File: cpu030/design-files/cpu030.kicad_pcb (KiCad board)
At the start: 4 copper layers, 259.9 x 154.9 mm, 199 parts, among them J101 Reset, J102 SYSCTL JTAG, J103 NMI, J201 DRAM0SZ, J202 DRAM0 JTAG, J301 UART1 FTDI, J302 UART0 FTDI, J303 UART0, J304 UART1, J401 ISACTL JTAG, J501 ATA connector, J502 5V CF Power, J701 RJ45_Amphenol_RJMG1BD3B8K1ANR, J801 DIN41612_03x32_ABC, J901 ATX-24, SW101 Reset, SW102 NMI, U101 MC68030RC, U102 ATF1508AS, U103 MC74ACT05DG, U104 DS1813, U105 SST39SF040 (E), U106 SST39SF040 (O), U107 MC68882, U108 GAL22V10, U109 MC74ACT05DG, U110 DS1813, U201 ATF1508AS, U202 CY7C1061GE (U16), U203 CY7C1061GE (L16), U204 SIMM72-0A, U205 SIMM72-0B, U206 MC74ACT05DG, U301 TL16C2552, U401 ATF1508AS, U402 MC74ACT05DG, U501 74ACT245, U502 74ACT245, U503 74ACT245, U601 PCF8584, U602 DS3231MZ, U701 RTL8019AS, U702 AT93C46D-PU, U801 74ACT245, U802 74ACT245, U803 74ACT245, U804 74ACT245, U805 74ACT245, U806 74ACT245, U807 74ACT245, U808 74ACT245, Y101 50MHz, Y301 1.8432MHz, Y701 20MHz

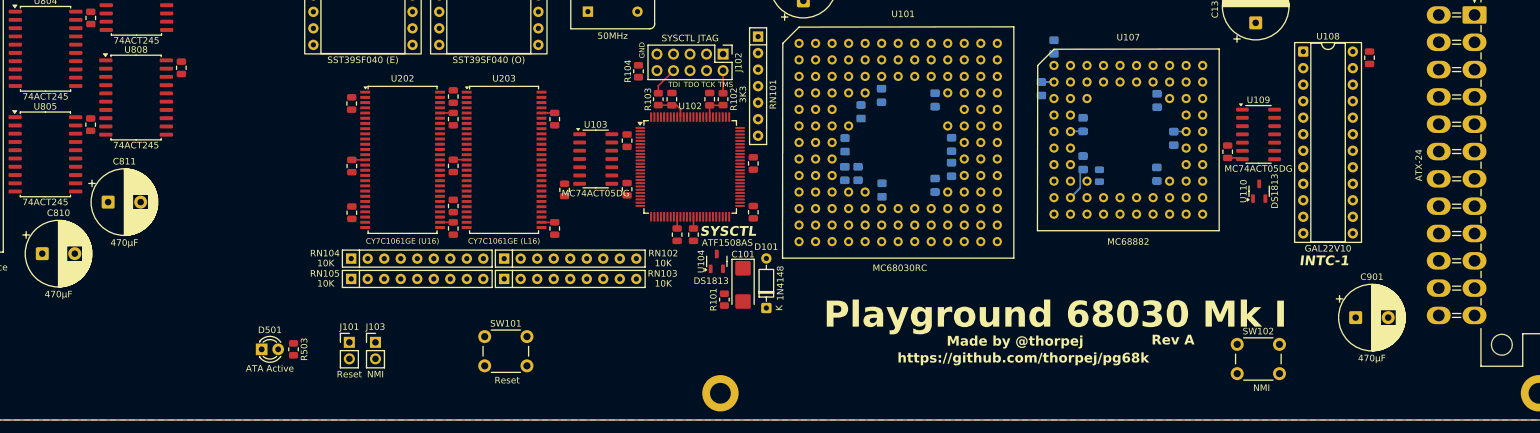
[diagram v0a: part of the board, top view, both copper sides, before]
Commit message: Manually route +12V and -12V.
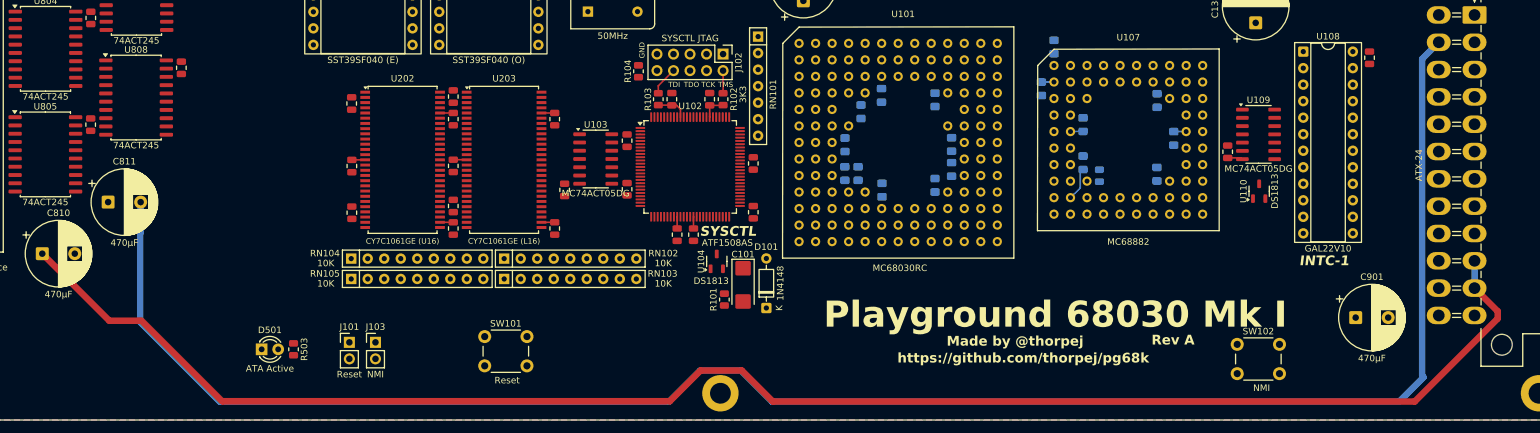
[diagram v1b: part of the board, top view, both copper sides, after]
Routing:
- net -12V: track 0.00 -> 279.0 mm
- net +12V: track 0.00 -> 252.5 mm
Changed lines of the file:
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@@
+	)
+	(segment
+		(start 224.2312 236.4994)
+		(end 219.4348 231.703)
+		(width 1)
+		(layer "B.Cu")
+		(net 429)
+	)
+	(segment
+		(start 139.2936 236.474)
+		(end 127.0762 224.2566)
+		(width 1)
+		(layer "B.Cu")
+		(net 429)
+	)
+	(segment
+		(start 324.172 232.5288)
+		(end 324.3834 232.7402)
+		(width 1)
+		(layer "B.Cu")
+		(net 429)
+	)
+	(segment
+		(start 127.143123 210.473677)
+		(end 127.143123 205.8162)
+		(width 1)
+		(layer "B.Cu")
+		(net 429)
+	)
+	(segment
+		(start 208.407 236.474)
+		(end 139.2936 236.474)
+		(width 1)
+		(layer "B.Cu")
+		(net 429)
+	)
+	(segment
+		(start 324.172 183.7916)
+		(end 324.172 232.5288)
+		(width 1)
+		(layer "B.Cu")
+		(net 429)
+	)
+	(segment
+		(start 127.0762 210.5406)
+		(end 127.143123 210.473677)
+		(width 1)
+		(layer "B.Cu")
+		(net 429)
+	)
+	(segment
+		(start 219.4348 231.703)
+		(end 213.178 231.703)
+		(width 1)
+		(layer "B.Cu")
+		(net 429)
+	)
+	(segment
+		(start 127.0762 224.2566)
+		(end 127.0762 210.5406)
+		(width 1)
+		(layer "B.Cu")
+		(net 429)
+	)
+	(segment
+		(start 213.178 231.703)
+		(end 208.407 236.474)
+		(width 1)
+		(layer "B.Cu")
+		(net 429)
+	)
+	(segment
+		(start 326.723 181.2406)
+		(end 324.172 183.7916)
+		(width 1)
+		(layer "B.Cu")
+		(net 429)
+	)
+	(segment
+		(start 320.6242 236.4994)
+		(end 224.2312 236.4994)
+		(width 1)
+		(layer "B.Cu")
+		(net 429)
+	)
+	(segment
+		(start 324.3834 232.7402)
+		(end 320.6242 236.4994)
+		(width 1)
+		(layer "B.Cu")
+		(net 429)
+	)
+	(segment
+		(start 127.1524 224.0534)
+		(end 122.3302 224.0534)
+		(width 1)
+		(layer "F.Cu")
+		(net 431)
+	)
+	(segment
+		(start 219.5618 231.703)
+		(end 213.2288 231.703)
+		(width 1)
+		(layer "F.Cu")
+		(net 431)
+	)
+	(segment
+		(start 335.7118 223.7994)
+		(end 323.0372 236.474)
+		(width 1)
+		(layer "F.Cu")
+		(net 431)
+	)
+	(segment
+		(start 208.5086 236.4232)
+		(end 139.7508 236.4232)
+		(width 1)
+		(layer "F.Cu")
+		(net 431)
+	)
+	(segment
+		(start 224.3328 236.474)
+		(end 219.5618 231.703)
+		(width 1)
+		(layer "F.Cu")
+		(net 431)
+	)
+	(segment
+		(start 335.788 222.6056)
+		(end 335.788 223.7232)
+		(width 1)
+		(layer "F.Cu")
+		(net 431)
+	)
+	(segment
+		(start 213.2288 231.703)
+		(end 208.5086 236.4232)
+		(width 1)
+		(layer "F.Cu")
+		(net 431)
+	)
+	(segment
+		(start 323.0372 236.474)
+		(end 224.3328 236.474)
+		(width 1)
+		(layer "F.Cu")
+		(net 431)
+	)
+	(segment
+		(start 139.7 236.474)
+		(end 127.2794 224.0534)
+		(width 1)
+		(layer "F.Cu")
+		(net 431)
+	)
+	(segment
+		(start 122.3302 224.0534)
+		(end 112.0178 213.741)
+		(width 1)
+		(layer "F.Cu")
+		(net 431)
+	)
+	(segment
+		(start 332.223 219.0406)
+		(end 335.788 222.6056)
+		(width 1)
+		(layer "F.Cu")
+		(net 431)
+	)
+	(segment
+		(start 332.223 214.8406)
+		(end 332.223 219.0406)
+		(width 1)
+		(layer "B.Cu")
+		(net 431)
 	)
 	(segment
